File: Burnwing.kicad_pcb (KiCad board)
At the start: 4 copper layers, 50.8 x 22.9 mm, 49 parts, among them J1 USB Type C, J2 Conn_01x06_MountingPin, J4 Conn_01x04_Pin, Q2 AONR21307, SW1 SW_DIP_x02, U1 HUSB238, U2 BTS7030-2EPA

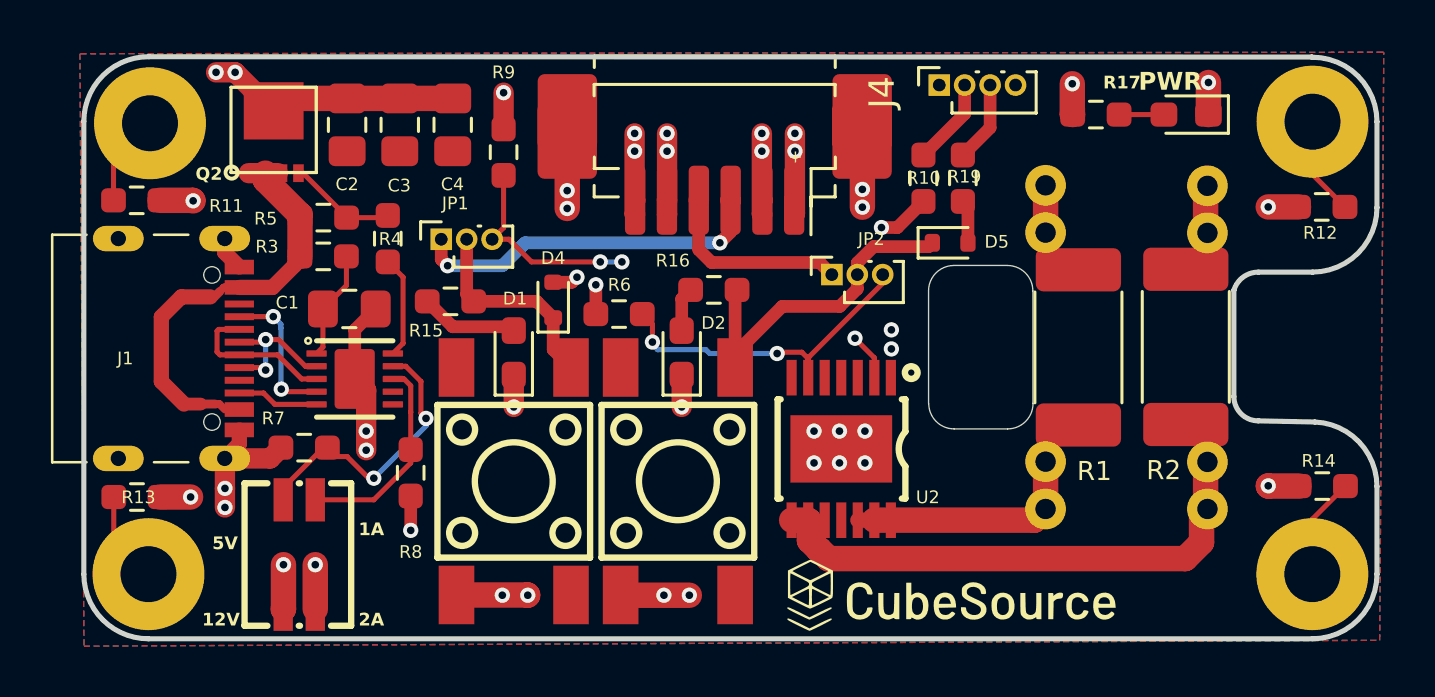
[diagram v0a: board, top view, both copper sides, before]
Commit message: Fixed VDC traces
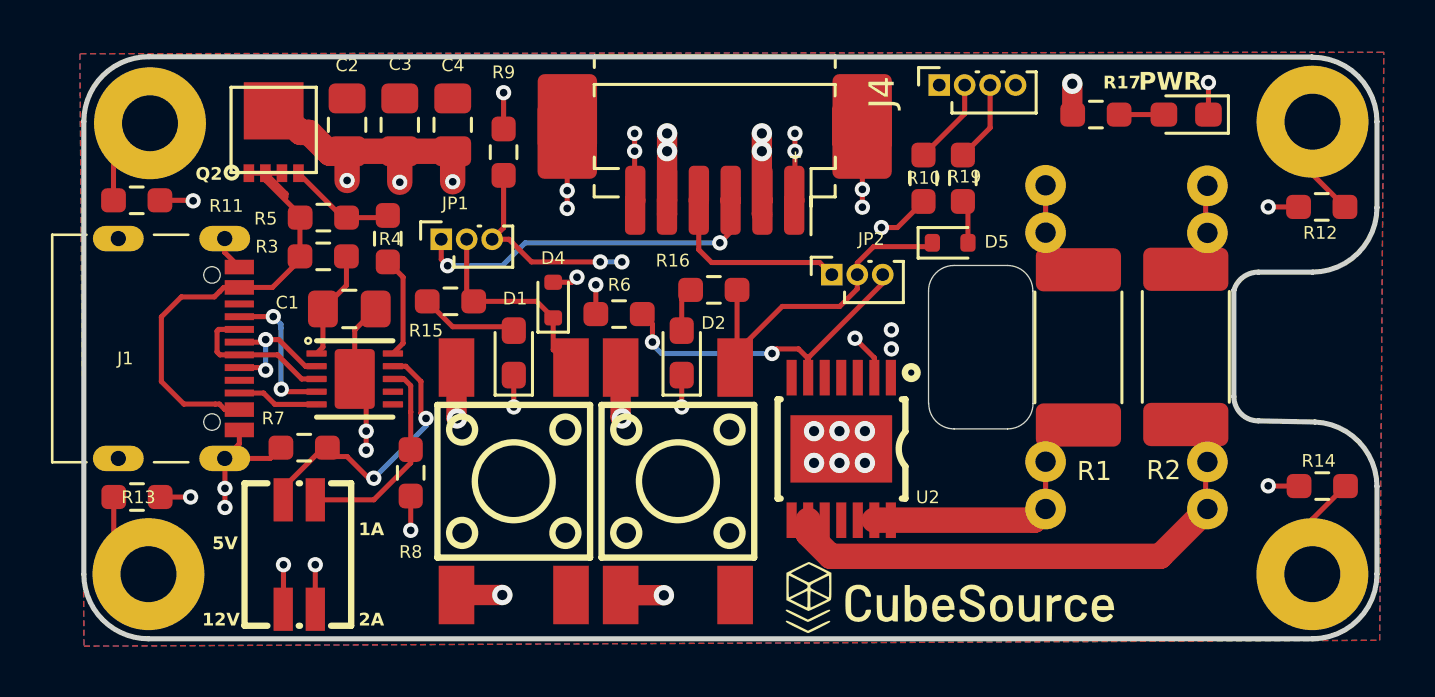
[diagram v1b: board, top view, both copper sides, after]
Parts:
- moved .space 0.11 mm to (111.2, 101.4)
- turned C2 to 90 degrees
- turned C3 to 90 degrees
- turned C4 to 90 degrees
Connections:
- Burn1 pad 3: Net-(Burn1-C) -> (no net)
- Burn2 pad 3: Net-(Burn2-C) -> (no net)
- C2 pad 2: Net-(C2-Pad2) -> GND
- C3 pad 2: Net-(C2-Pad2) -> GND
- C4 pad 2: Net-(C2-Pad2) -> GND
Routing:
- net VDC: track 23.3 -> 27.2 mm, vias 17 -> 18
- net GND: track 44.9 -> 48.3 mm
- net Net-(R2-Pad2): track 22.3 -> 21.0 mm
- net Net-(Burn2-C): track 14.8 -> 13.8 mm
- net Net-(R1-Pad2): track 11.1 -> 10.5 mm
